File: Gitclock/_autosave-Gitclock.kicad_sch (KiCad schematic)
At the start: 46 parts, among them J1 PJ-102AH, J2 Conn_01x06, SW1 Omron_B3F_SPST, SW5 RotaryEncoder_Switch, U1 ATmega328-PU, U2 L7805, U3 MAX7219, U4 DS1307_DIP-8, Y1 Crystal_16MHz, Y2 Crystal_32768Hz

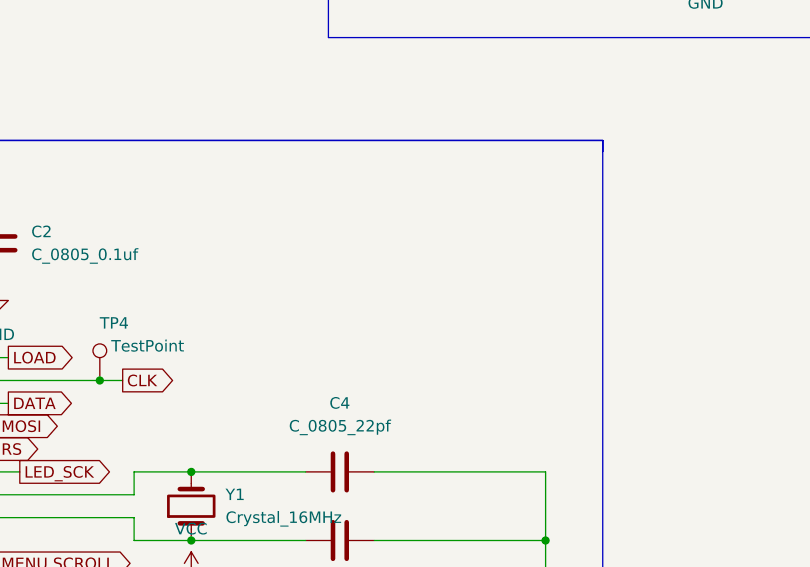
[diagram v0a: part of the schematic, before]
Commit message: clock_complete
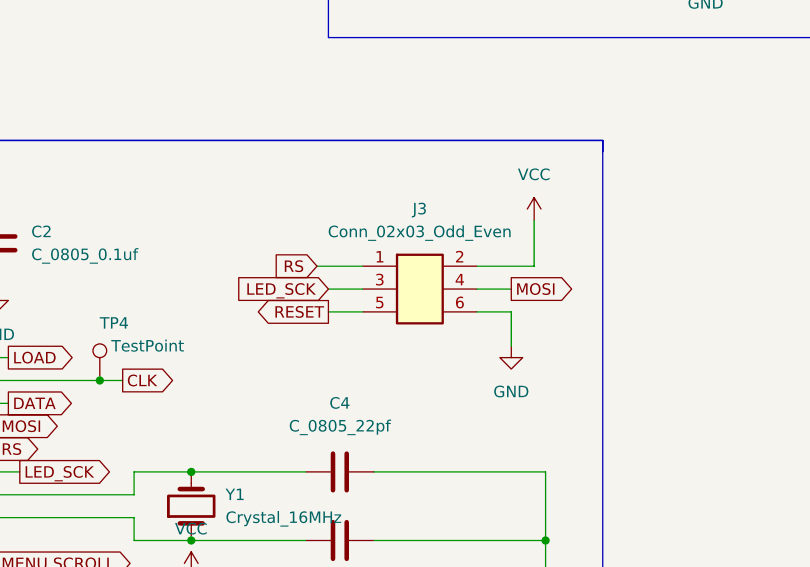
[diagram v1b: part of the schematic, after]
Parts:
- added J3: Conn_02x03_Odd_Even, footprints:PinHeader_2x03_P2.54mm_Vertical, symbol HPS:Conn_02x03_Odd_Even
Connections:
- net GND: now also J3.6 (Pin_6)
- net LED_SCK: now also J3.3 (Pin_3)
- net MOSI: now also J3.4 (Pin_4)
- net RESET: now also J3.5 (Pin_5)
- net RS: now also J3.1 (Pin_1)
- net VCC: now also J3.2 (Pin_2)
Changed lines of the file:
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@@
+    (stroke (width 0) (type default) (color 0 0 0 0))
+  )
+  (wire (pts (xy 251.46 114.3) (xy 255.27 114.3))
     (stroke (width 0) (type default) (color 0 0 0 0))
   )
@@
     (stroke (width 0) (type default) (color 0 0 0 0))
   )
+  (wire (pts (xy 251.46 116.84) (xy 255.27 116.84))
+    (stroke (width 0) (type default) (color 0 0 0 0))
+  )
   (polyline (pts (xy 265.43 97.79) (xy 265.43 201.93))
     (stroke (width 0) (type default) (color 0 0 0 0))
@@
     (stroke (width 0) (type default) (color 0 0 0 0))
   )
+  (wire (pts (xy 255.27 116.84) (xy 255.27 120.65))
+    (stroke (width 0) (type default) (color 0 0 0 0))
+  )
   (polyline (pts (xy 229.87 26.67) (xy 229.87 81.28))
     (stroke (width 0) (type default) (color 0 0 0 0))
@@
     (stroke (width 0) (type default) (color 0 0 0 0))
   )
+  (wire (pts (xy 233.68 111.76) (xy 238.76 111.76))
+    (stroke (width 0) (type default) (color 0 0 0 0))
+  )
   (wire (pts (xy 50.8 121.92) (xy 50.8 127))
     (stroke (width 0) (type default) (color 0 0 0 0))
@@
     (stroke (width 0) (type default) (color 0 0 0 0))
   )
+  (wire (pts (xy 257.81 111.76) (xy 257.81 106.68))
+    (stroke (width 0) (type default) (color 0 0 0 0))
+  )
   (polyline (pts (xy 106.68 143.51) (xy 106.68 193.04))
     (stroke (width 0) (type default) (color 0 0 0 0))
@@
     (stroke (width 0) (type default) (color 0 0 0 0))
   )
+  (wire (pts (xy 234.95 114.3) (xy 238.76 114.3))
+    (stroke (width 0) (type default) (color 0 0 0 0))
+  )
   (wire (pts (xy 182.88 110.49) (xy 182.88 114.3))
     (stroke (width 0) (type default) (color 0 0 0 0))
@@
     (stroke (width 0) (type default) (color 0 0 0 0))
   )
+  (wire (pts (xy 234.95 116.84) (xy 238.76 116.84))
+    (stroke (width 0) (type default) (color 0 0 0 0))
+  )
   (wire (pts (xy 29.21 71.12) (xy 30.48 71.12))
+    (stroke (width 0) (type default) (color 0 0 0 0))
+  )
+  (wire (pts (xy 251.46 111.76) (xy 257.81 111.76))
     (stroke (width 0) (type default) (color 0 0 0 0))
   )
@@
     )
   )
+  (global_label "RESET" (shape output) (at 234.95 116.84 180) (fields_autoplaced)
+    (effects (font (size 1.27 1.27)) (justify right))
+    (property "Intersheet References" "${INTERSHEET_REFS}" (id 0) (at 226.7917 116.7606 0)
+      (effects (font (size 1.27 1.27)) (justify right) hide)
+    )
+  )
   (global_label "MENU_B" (shape output) (at 198.12 152.4 0) (fields_autoplaced)
     (effects (font (size 1.27 1.27)) (justify left))
@@
     (property "Intersheet References" "${INTERSHEET_REFS}" (id 0) (at 206.2179 126.9206 0)
       (effects (font (size 1.27 1.27)) (justify left) hide)
+    )
+  )
+  (global_label "LED_SCK" (shape input) (at 234.95 114.3 180) (fields_autoplaced)
+    (effects (font (size 1.27 1.27)) (justify right))
+    (property "Intersheet References" "${INTERSHEET_REFS}" (id 0) (at 224.3726 114.2206 0)
+      (effects (font (size 1.27 1.27)) (justify right) hide)
     )
   )
@@
     )
   )
+  (global_label "MOSI" (shape output) (at 255.27 114.3 0) (fields_autoplaced)
+    (effects (font (size 1.27 1.27)) (justify left))
+    (property "Intersheet References" "${INTERSHEET_REFS}" (id 0) (at 262.2793 114.2206 0)
+      (effects (font (size 1.27 1.27)) (justify left) hide)
+    )
+  )
   (global_label "MENU_B" (shape input) (at 389.89 68.58 0) (fields_autoplaced)
     (effects (font (size 1.27 1.27)) (justify left))
@@
     (property "Intersheet References" "${INTERSHEET_REFS}" (id 0) (at 243.4107 157.4006 0)
       (effects (font (size 1.27 1.27)) (justify left) hide)
+    )
+  )
+  (global_label "RS" (shape input) (at 233.68 111.76 180) (fields_autoplaced)
+    (effects (font (size 1.27 1.27)) (justify right))
+    (property "Intersheet References" "${INTERSHEET_REFS}" (id 0) (at 228.7874 111.6806 0)
+      (effects (font (size 1.27 1.27)) (justify right) hide)
     )
   )
@@
     )
     (property "Datasheet" "" (id 3) (at 118.11 137.16 0)
+      (effects (font (size 1.27 1.27)) hide)
+    )
+    (pin "1")
+  )
+  (symbol (lib_id "HPS:VCC") (at 257.81 106.68 0) (unit 1)
+    (in_bom yes) (on_board yes) (fields_autoplaced)
+    (property "Reference" "#PWR012" (id 0) (at 257.81 110.49 0)
+      (effects (font (size 1.27 1.27)) hide)
+    )
+    (property "Value" "VCC" (id 1) (at 257.81 101.6 0))
+    (property "Footprint" "" (id 2) (at 257.81 106.68 0)
+      (effects (font (size 1.27 1.27)) hide)
+    )
+    (property "Datasheet" "" (id 3) (at 257.81 106.68 0)
       (effects (font (size 1.27 1.27)) hide)
     )
@@
     )
     (property "Datasheet" "~" (id 3) (at 214.63 124.46 0)
+      (effects (font (size 1.27 1.27)) hide)
+    )
+    (pin "1")
+  )
+  (symbol (lib_id "HPS:GND") (at 255.27 120.65 0) (unit 1)
+    (in_bom yes) (on_board yes) (fields_autoplaced)
+    (property "Reference" "#PWR011" (id 0) (at 255.27 127 0)
+      (effects (font (size 1.27 1.27)) hide)
+    )
+    (property "Value" "GND" (id 1) (at 255.27 125.73 0))
+    (property "Footprint" "" (id 2) (at 255.27 120.65 0)
+      (effects (font (size 1.27 1.27)) hide)
+    )
+    (property "Datasheet" "" (id 3) (at 255.27 120.65 0)
       (effects (font (size 1.27 1.27)) hide)
     )
@@
     (pin "9")
   )
+  (symbol (lib_id "HPS:Conn_02x03_Odd_Even") (at 245.11 115.57 0) (unit 1)
+    (in_bom yes) (on_board yes) (fields_autoplaced)
+    (property "Reference" "J3" (id 0) (at 245.11 105.41 0))
+    (property "Value" "Conn_02x03_Odd_Even" (id 1) (at 245.11 107.95 0))
+    (property "Footprint" "footprints:PinHeader_2x03_P2.54mm_Vertical" (id 2) (at 245.11 127 0)
+      (effects (font (size 1.27 1.27)) hide)
+    )
+    (property "Datasheet" "https://drawings-pdf.s3.amazonaws.com/11636.pdf" (id 3) (at 243.84 116.84 0)
+      (effects (font (size 1.27 1.27)) hide)
+    )
+    (property "MFG" "Sullins Connector Solutions" (id 4) (at 245.11 121.92 0)
+      (effects (font (size 1.27 1.27)) hide)
+    )
+    (property "MPN" "PRPC003DAAN-RC" (id 5) (at 245.11 124.46 0)
+      (effects (font (size 1.27 1.27)) hide)
+    )
+    (property "Digikey PN" "S2011EC-03-ND" (id 6) (at 245.11 129.54 0)
+      (effects (font (size 1.27 1.27)) hide)
+    )
+    (property "Mouser PN" "N/A" (id 7) (at 245.11 132.08 0)
+      (effects (font (size 1.27 1.27)) hide)
+    )
+    (pin "1")
+    (pin "2")
+    (pin "3")
+    (pin "4")
+    (pin "5")
+    (pin "6")
+  )
   (symbol (lib_id "HPS:C_0805_22pf") (at 236.22 142.24 90) (unit 1)
     (in_bom yes) (on_board yes)
@@
       (reference "#PWR010") (unit 1) (value "GND") (footprint "")
     )
+    (path "/58dfc7d5-799d-426e-8f3c-66cf9649ac97"
+      (reference "#PWR011") (unit 1) (value "GND") (footprint "")
+    )
+    (path "/4ab19e56-beb2-4b95-bf72-08a88f175791"
+      (reference "#PWR012") (unit 1) (value "VCC") (footprint "")
+    )
     (path "/28b58255-5998-4ed5-b0e6-f11621736c10"
       (reference "#PWR013") (unit 1) (value "GND") (footprint "")
@@
       (reference "J2") (unit 1) (value "Conn_01x06") (footprint "footprints:PinHeader_1x06_P2.54mm_Vertical")
     )
+    (path "/8442304a-cdc3-4f8a-93f6-f80d75de7e98"
+      (reference "J3") (unit 1) (value "Conn_02x03_Odd_Even") (footprint "footprints:PinHeader_2x03_P2.54mm_Vertical")
+    )
     (path "/e97dfe19-02c8-4781-ad7b-2aea401b9af7"
